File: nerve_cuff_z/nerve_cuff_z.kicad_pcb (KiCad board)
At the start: 2 copper layers, 4 x 5.7 mm, 4 parts

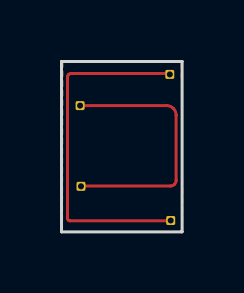
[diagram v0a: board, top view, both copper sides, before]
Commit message: all boards cleaned up + passing DRC
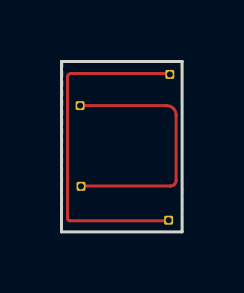
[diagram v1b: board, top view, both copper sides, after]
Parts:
- moved REF** 0.07 mm to (103.5, 70.2)
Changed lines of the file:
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@@
   (net 0 "")
   (footprint "nerve_cuff_pad:solder_wire_pad" (layer "F.Cu")
-    (at 103.6 70.22)
+    (at 103.53 70.21)
     (descr "Soldered wire connection, for a single 0.1 mm² wire, basic insulation, conductor diameter 0.4mm, outer diameter 1mm, size source Multi-Contact FLEXI-E 0.1 (https://ec.staubli.com/AcroFiles/Catalogues/TM_Cab-Main-11014119_(en)_hi.pdf), bend radius 3 times outer diameter, generated with kicad-footprint-generator")
     (tags "connector wire 0.1sqmm")
@@
         (effects (font (size 1 1) (thickness 0.15)))
     )
-    (fp_line (start -0.2 -0.2) (end -0.2 0.2)
+    (fp_line (start -0.3 -0.3) (end -0.3 0.3)
       (stroke (width 0.05) (type solid)) (layer "F.CrtYd"))
-    (fp_line (start -0.2 0.2) (end 0.2 0.2)
+    (fp_line (start -0.3 0.3) (end 0.3 0.3)
       (stroke (width 0.05) (type solid)) (layer "F.CrtYd"))
-    (fp_line (start 0.2 -0.2) (end -0.2 -0.2)
+    (fp_line (start 0.3 -0.3) (end -0.3 -0.3)
       (stroke (width 0.05) (type solid)) (layer "F.CrtYd"))
-    (fp_line (start 0.2 0.2) (end 0.2 -0.2)
+    (fp_line (start 0.3 0.3) (end 0.3 -0.3)
       (stroke (width 0.05) (type solid)) (layer "F.CrtYd"))
     (pad "1" thru_hole roundrect (at 0 0) (size 0.3 0.3) (drill 0.2) (layers "*.Cu" "*.Mask") (roundrect_rratio 0.15625))
@@
         (effects (font (size 1 1) (thickness 0.15)))
     )
-    (fp_line (start -0.2 -0.2) (end -0.2 0.2)
+    (fp_line (start -0.3 -0.3) (end -0.3 0.3)
       (stroke (width 0.05) (type solid)) (layer "F.CrtYd"))
-    (fp_line (start -0.2 0.2) (end 0.2 0.2)
+    (fp_line (start -0.3 0.3) (end 0.3 0.3)
       (stroke (width 0.05) (type solid)) (layer "F.CrtYd"))
-    (fp_line (start 0.2 -0.2) (end -0.2 -0.2)
+    (fp_line (start 0.3 -0.3) (end -0.3 -0.3)
       (stroke (width 0.05) (type solid)) (layer "F.CrtYd"))
-    (fp_line (start 0.2 0.2) (end 0.2 -0.2)
+    (fp_line (start 0.3 0.3) (end 0.3 -0.3)
       (stroke (width 0.05) (type solid)) (layer "F.CrtYd"))
     (pad "1" thru_hole roundrect (at 0 0) (size 0.3 0.3) (drill 0.2) (layers "*.Cu" "*.Mask") (roundrect_rratio 0.15625))
@@
         (effects (font (size 1 1) (thickness 0.15)))
     )
-    (fp_line (start -0.2 -0.2) (end -0.2 0.2)
+    (fp_line (start -0.3 -0.3) (end -0.3 0.3)
       (stroke (width 0.05) (type solid)) (layer "F.CrtYd"))
-    (fp_line (start -0.2 0.2) (end 0.2 0.2)
+    (fp_line (start -0.3 0.3) (end 0.3 0.3)
       (stroke (width 0.05) (type solid)) (layer "F.CrtYd"))
-    (fp_line (start 0.2 -0.2) (end -0.2 -0.2)
+    (fp_line (start 0.3 -0.3) (end -0.3 -0.3)
       (stroke (width 0.05) (type solid)) (layer "F.CrtYd"))
-    (fp_line (start 0.2 0.2) (end 0.2 -0.2)
+    (fp_line (start 0.3 0.3) (end 0.3 -0.3)
       (stroke (width 0.05) (type solid)) (layer "F.CrtYd"))
     (pad "1" thru_hole roundrect (at 0 0) (size 0.3 0.3) (drill 0.2) (layers "*.Cu" "*.Mask") (roundrect_rratio 0.15625))
@@
         (effects (font (size 1 1) (thickness 0.15)))
     )
-    (fp_line (start -0.2 -0.2) (end -0.2 0.2)
+    (fp_line (start -0.3 -0.3) (end -0.3 0.3)
       (stroke (width 0.05) (type solid)) (layer "F.CrtYd"))
-    (fp_line (start -0.2 0.2) (end 0.2 0.2)
+    (fp_line (start -0.3 0.3) (end 0.3 0.3)
       (stroke (width 0.05) (type solid)) (layer "F.CrtYd"))
-    (fp_line (start 0.2 -0.2) (end -0.2 -0.2)
+    (fp_line (start 0.3 -0.3) (end -0.3 -0.3)
       (stroke (width 0.05) (type solid)) (layer "F.CrtYd"))
-    (fp_line (start 0.2 0.2) (end 0.2 -0.2)
+    (fp_line (start 0.3 0.3) (end 0.3 -0.3)
       (stroke (width 0.05) (type solid)) (layer "F.CrtYd"))
     (pad "1" thru_hole roundrect (at 0 0) (size 0.3 0.3) (drill 0.2) (layers "*.Cu" "*.Mask") (roundrect_rratio 0.15625))
@@
   )
   (dimension (type aligned) (layer "F.SilkS")
-    (pts (xy 103.98 64.92) (xy 103.98 70.6))
+    (pts (xy 103.3 65.29) (xy 103.3 70.97))
     (height -5.97)
-    (gr_text "5.6800 mm" (at 108.8 67.76 90) (layer "F.SilkS")
+    (gr_text "5.6800 mm" (at 108.12 68.13 90) (layer "F.SilkS")
       (effects (font (size 1 1) (thickness 0.15)))
     )
@@
     (style (thickness 0.15) (arrow_length 1.27) (text_position_mode 0) (extension_height 0.58642) (extension_offset 0.5) keep_text_aligned)
   )
-  (segment (start 100.245355 70.23) (end 103.58 70.23) (width 0.1) (layer "F.Cu") (net 0))
+  (segment (start 100.245355 70.23) (end 103.51 70.23) (width 0.1) (layer "F.Cu") (net 0))
   (segment (start 103.78 68.882218) (end 103.78 66.708293) (width 0.1) (layer "F.Cu") (net 0))
+  (segment (start 103.54 65.32) (end 100.279497 65.32) (width 0.1) (layer "F.Cu") (net 0))
   (segment (start 100.16 65.439497) (end 100.16 70.144644) (width 0.1) (layer "F.Cu") (net 0))
-  (segment (start 103.54 65.32) (end 100.279497 65.32) (width 0.1) (layer "F.Cu") (net 0))
   (segment (start 103.592218 69.07) (end 100.59 69.07) (width 0.1) (layer "F.Cu") (net 0))
   (segment (start 103.461706 66.39) (end 100.58 66.39) (width 0.1) (layer "F.Cu") (net 0))
-  (segment (start 103.58 70.23) (end 103.63 70.18) (width 0.1) (layer "F.Cu") (net 0))
-  (arc (start 100.279497 65.32) (mid 100.233768 65.329096) (end 100.195 65.355) (width 0.1) (layer "F.Cu") (net 0))
   (arc (start 103.78 68.882218) (mid 103.765705 68.954079) (end 103.725 69.015) (width 0.1) (layer "F.Cu") (net 0))
+  (arc (start 100.195 65.355) (mid 100.169096 65.393767) (end 100.16 65.439497) (width 0.1) (layer "F.Cu") (net 0))
+  (arc (start 100.185 70.205) (mid 100.212691 70.223508) (end 100.245355 70.23) (width 0.1) (layer "F.Cu") (net 0))
   (arc (start 103.686774 66.483226) (mid 103.583512 66.414228) (end 103.461706 66.39) (width 0.1) (layer "F.Cu") (net 0))
   (arc (start 103.725 69.015) (mid 103.664079 69.055705) (end 103.592218 69.07) (width 0.1) (layer "F.Cu") (net 0))
   (arc (start 103.686774 66.483226) (mid 103.755771 66.586487) (end 103.78 66.708293) (width 0.1) (layer "F.Cu") (net 0))
   (arc (start 100.16 70.144644) (mid 100.166497 70.177308) (end 100.185 70.205) (width 0.1) (layer "F.Cu") (net 0))
-  (arc (start 100.185 70.205) (mid 100.212691 70.223496) (end 100.245355 70.23) (width 0.1) (layer "F.Cu") (net 0))
-  (arc (start 100.195 65.355) (mid 100.169096 65.393767) (end 100.16 65.439497) (width 0.1) (layer "F.Cu") (net 0))
+  (arc (start 100.279497 65.32) (mid 100.233768 65.329096) (end 100.195 65.355) (width 0.1) (layer "F.Cu") (net 0))
   (zone (net 0) (net_name "") (layer "F.Cu") (hatch edge 0.1)
     (connect_pads (clearance 0.05))
